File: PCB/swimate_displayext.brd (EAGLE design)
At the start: 50.9 x 51.2 mm, 56 parts, among them IC1 LPC11U24, J1 FTSH-105-01-L-DV, T1 BSS84, T2 BSS84, U1 USD-SOCKETNEW, U3 NC7SV86P5X, U5 DS3231MZ/V+T, U6 MAX1595EUA33+, U7 MAX1811ESA-T, U8 MAX16054AZT+T, U9 HC_05, Y1 12.000MHz

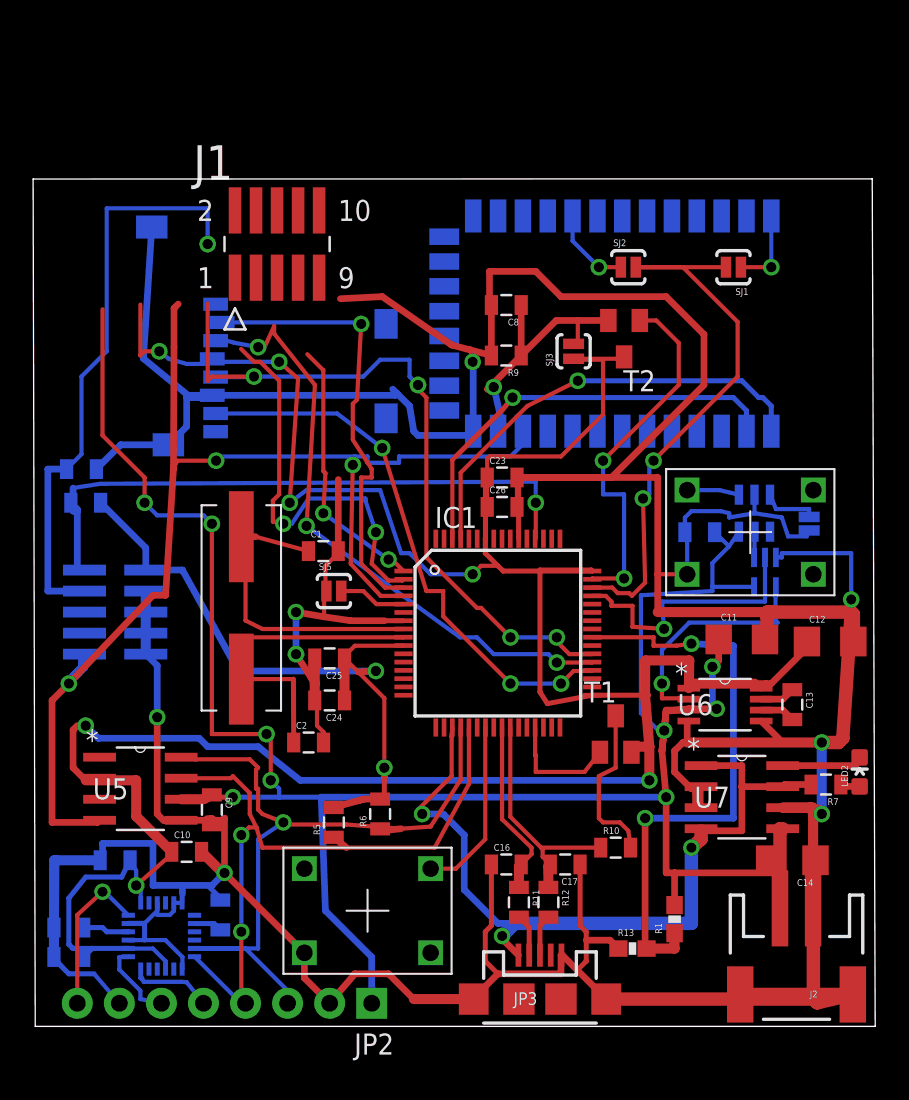
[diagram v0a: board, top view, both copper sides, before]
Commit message: Added top and bottom ground and power planes
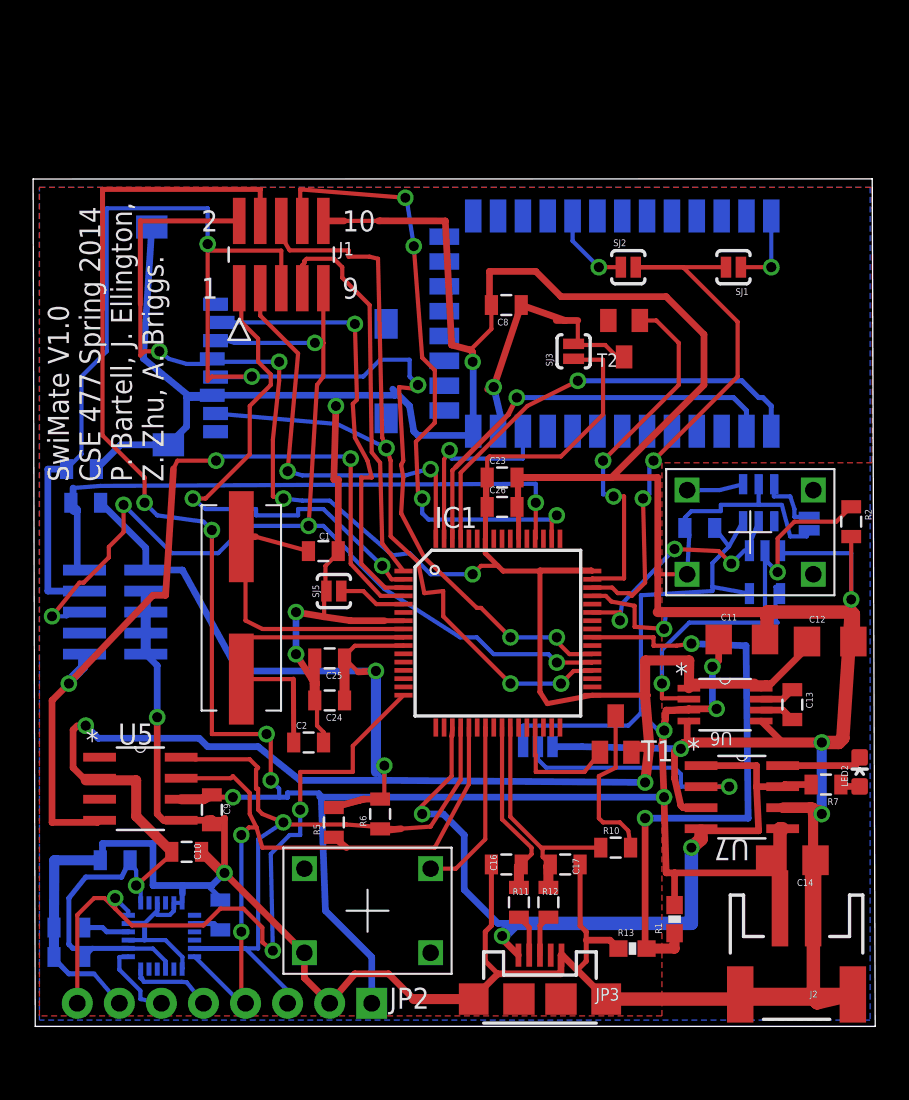
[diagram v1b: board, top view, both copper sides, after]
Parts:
- removed R9: 24K, SparkFun-Passives:0805
- added R2: 24k, SparkFun-Passives:0805
- added SJ6: (no value), SparkFun-Passives:SJ_3
- U3: value NC7SV86P5X -> NC7SZ32M5; device Fairchild_By_element14_Batch_1:SOT65P210X110-5N -> Fairchild_By_element14_Batch_1:SOT95P280X145-5N
- moved U8 0.68 mm to (43.7, 31.2)
- moved J1 0.68 mm to (14.9, 46.2)
- moved C15 0.25 mm to (40.1, 29.7)
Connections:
- removed net N$2: U3.1, U8.5
- removed net SPI_MOSI0: JTAG1.6
- new net BT_RST: IC1.63, U9.11
- new net DISP_RST: IC1.64, J1.3
- new net DISP_SW: IC1.50, J1.8
- new net N$3: SJ6.2, U7.2
- new net SW_PWR_STATE: IC1.43, U3.1, U8.5
- net 3.3V: now also T2.2; no longer T2.3
- net DISP_CS: now also IC1.1; no longer IC1.2
- net DISP_DC: now also IC1.2; no longer IC1.1
- net GND: now also R2.2, SJ6.1; no longer J1.8, R9.2, U7.2
- net MPU_INT: now also IC1.16
- net N$15: now also T2.3; no longer R9.1, T2.2
- net PO_DISABLE: now also R2.1
- net RST: no longer J1.3, U9.11
- net SPI0_MOSI: now also JTAG1.6
- net VBAT: now also SJ6.3
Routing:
- net DISP_SW: track 0.00 -> 38.2 mm, vias 0 -> 4
- net MPU_INT: track 9.71 -> 43.2 mm, vias 1 -> 3
- net VBAT: track 138.3 -> 166.0 mm
- net SPI0_MOSI: track 37.5 -> 65.0 mm, vias 3 -> 5
- net DISP_RST: track 0.00 -> 25.2 mm, vias 0 -> 2
- net GND: track 375.2 -> 398.3 mm, vias 8 -> 10
- net RST: track 75.8 -> 53.9 mm
- net SPI0_MISO: track 33.4 -> 53.1 mm
- net DISP_DC: track 16.1 -> 32.5 mm
- net N$3: track 0.00 -> 15.2 mm, vias 0 -> 1
- net SW_PWR_STATE: track 0.00 -> 14.8 mm, vias 0 -> 3
- net BT_RST: track 0.00 -> 12.2 mm, vias 0 -> 1
- net SPI0_SCK: track 80.8 -> 92.7 mm
- net PO_DISABLE: track 16.6 -> 25.4 mm, vias 1 -> 2
- net 3.3V: track 226.0 -> 232.1 mm
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- added copper zone on layer 1, net 3.3V
- added copper zone on layer 16, net GND
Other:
- board text added: "SwiMate V1.0 CSE 477 Spring 2014 P. Bartell, J. Ellington, Z. Zhu, A. Briggs."

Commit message: Final version of both PCBs.. Send to OSHPark
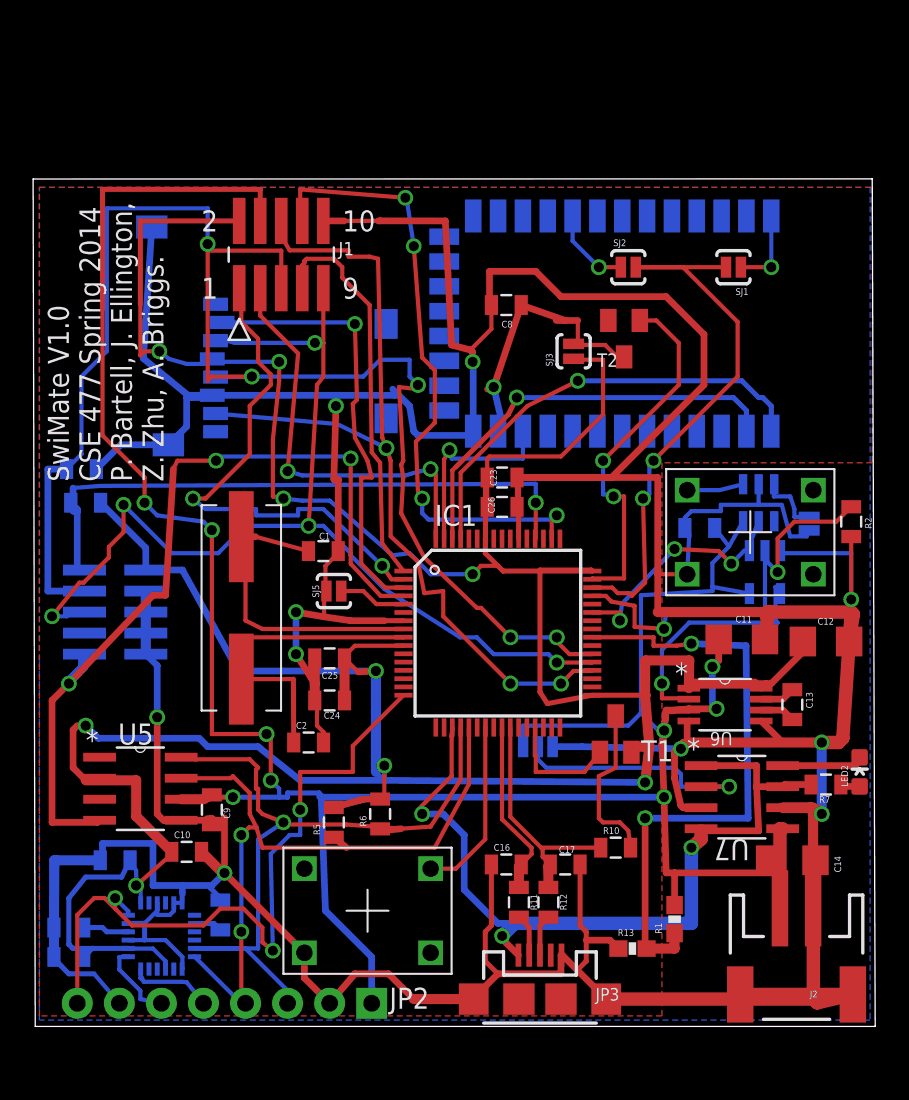
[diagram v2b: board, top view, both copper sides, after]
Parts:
- moved C12 0.25 mm to (47.8, 22.9)
